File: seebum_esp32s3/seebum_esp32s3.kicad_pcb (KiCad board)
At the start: 4 copper layers, 65 x 56 mm, 90 parts, among them J101 Conn_01x02_Pin, J102 Conn_01x04_Pin, J103 Conn_01x02_Pin, J201 USB_C_Receptacle_USB2.0_16P, J202 USB_C_Receptacle_USB2.0_16P, J203 Conn_02x10_Odd_Even, J204 Conn_02x10_Odd_Even, J401 GPIO, Q101 AO4407, Q201 UMH3N, SW101 SW_DPDT_x2, SW201 SW_MEC_5E, SW202 SW_MEC_5E, U201 ESP32-S3-WROOM-1, U202 CH343P, U203 AMS1117-3.3, U301 TPS56528

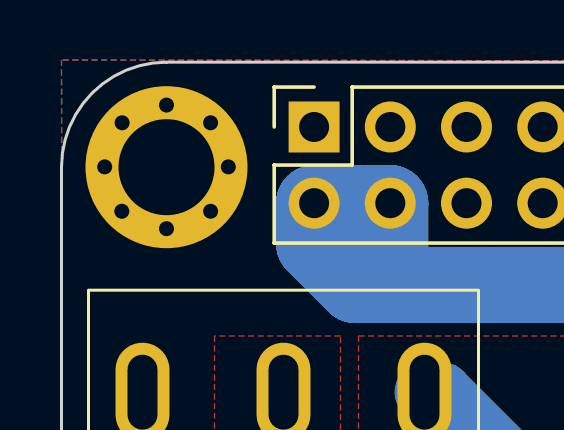
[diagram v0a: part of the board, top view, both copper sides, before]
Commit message: Feat: some improvments
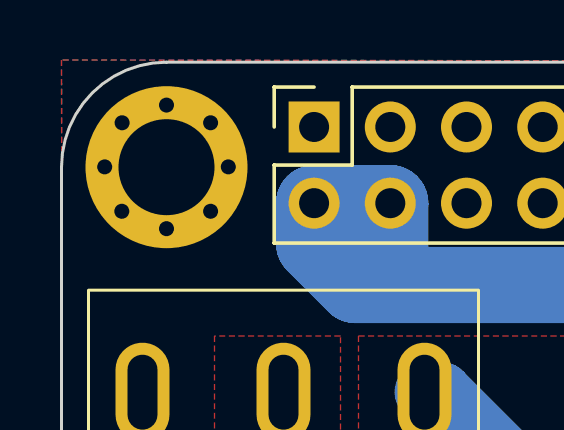
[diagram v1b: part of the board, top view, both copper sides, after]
